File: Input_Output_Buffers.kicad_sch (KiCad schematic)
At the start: 35 parts, among them J1 Conn_02x07_Odd_Even, J4 Conn_02x07_Odd_Even, U1 74HC245, U2 74HC245, U26 74HC245, U27 74HC245

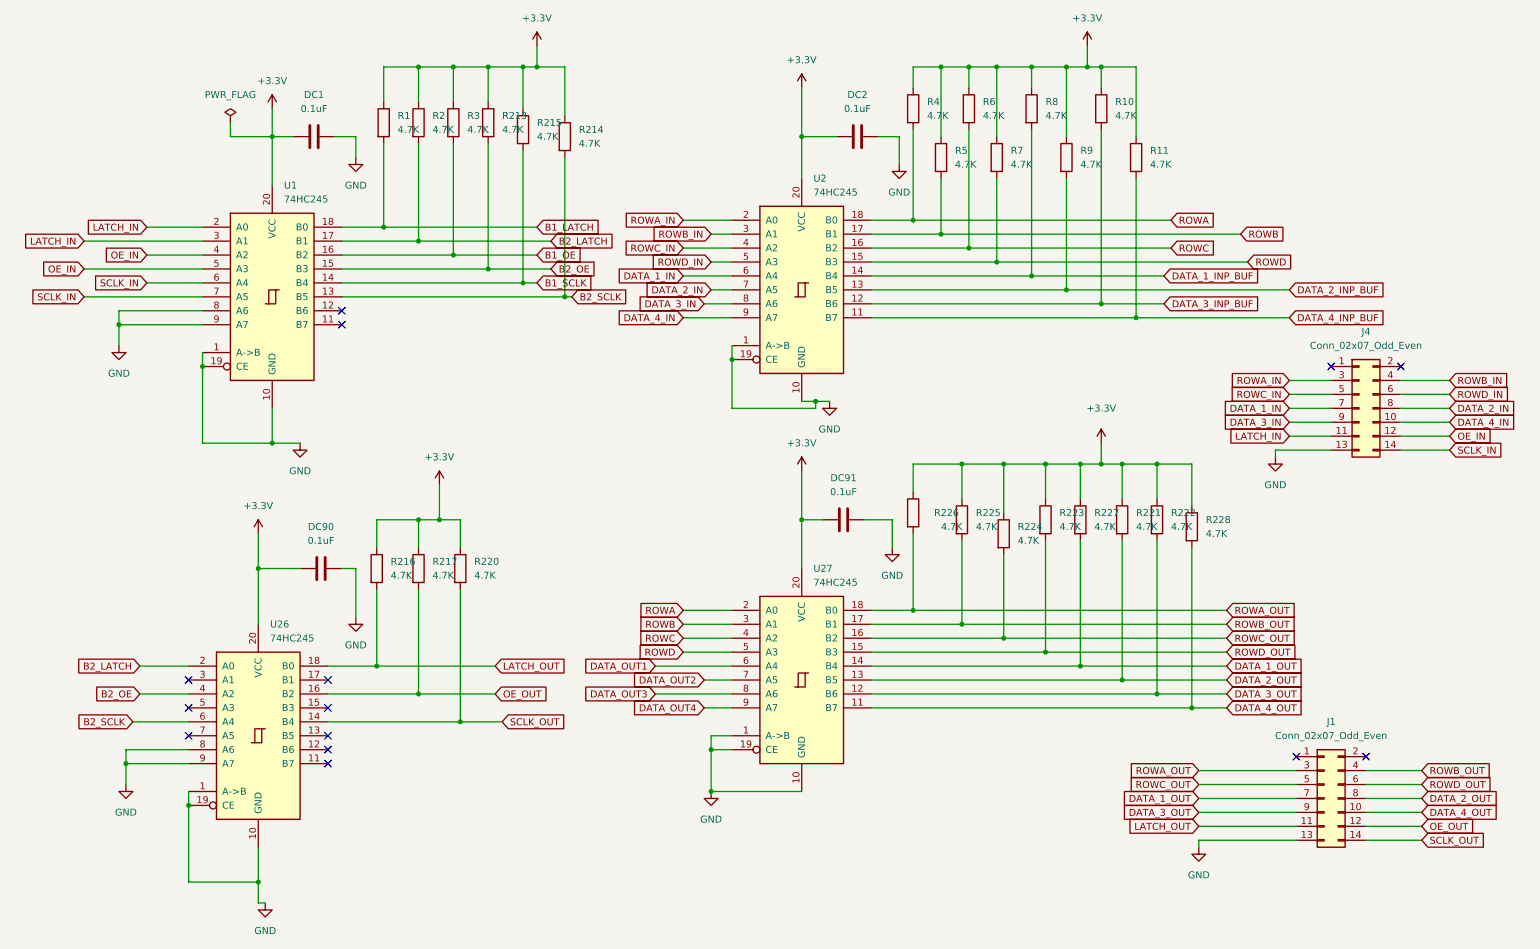
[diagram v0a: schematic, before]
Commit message: Updated PCB
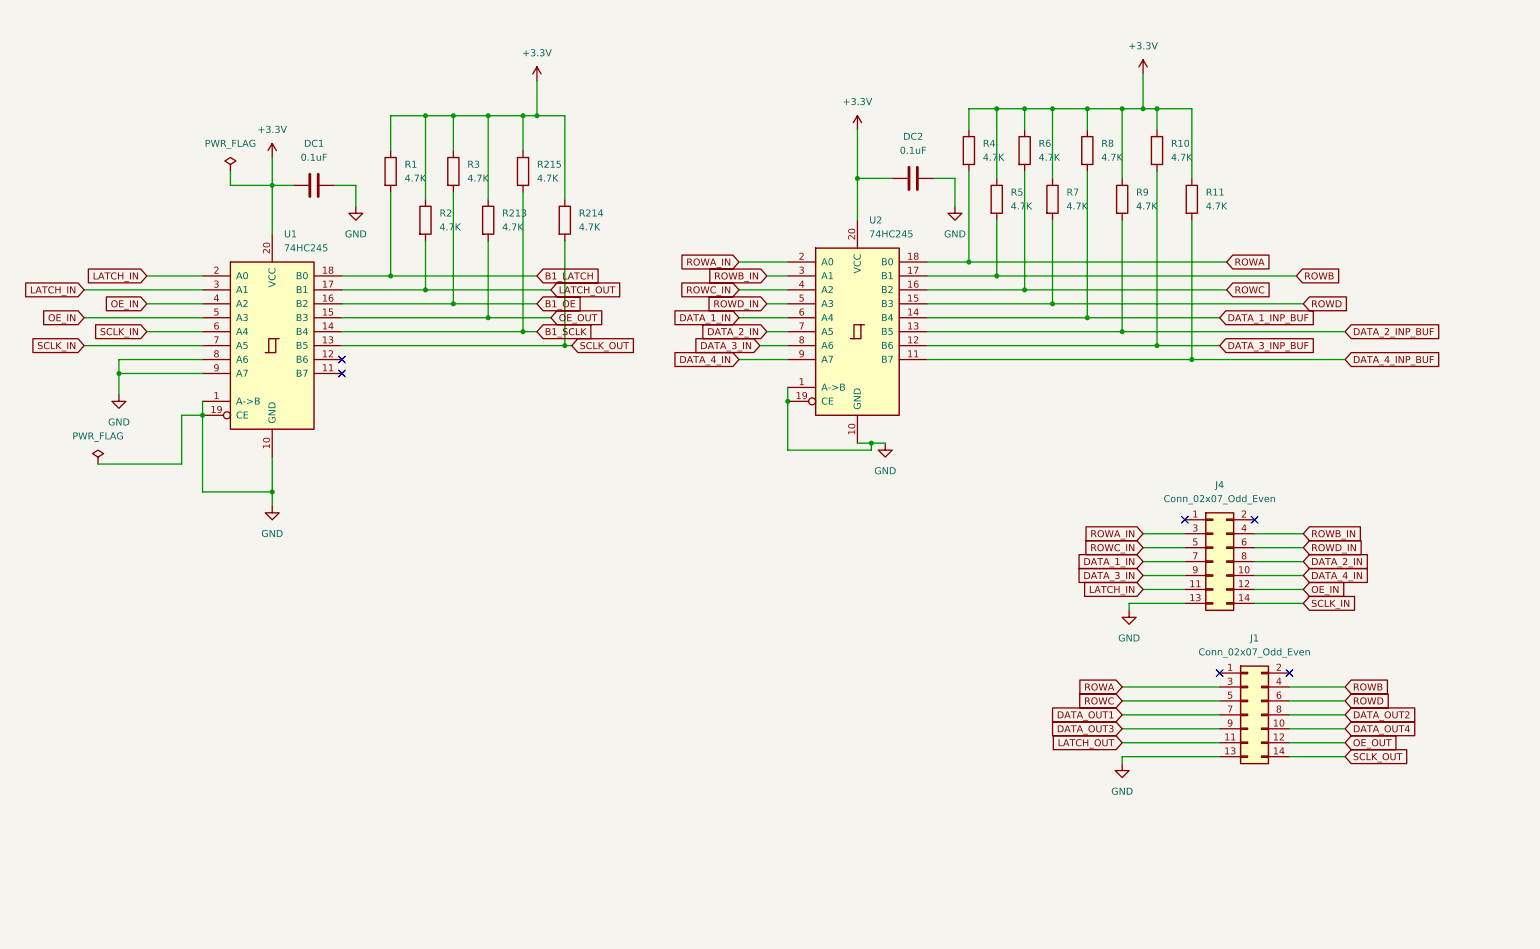
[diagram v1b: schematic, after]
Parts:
- removed DC90, DC91: 0.1uF, Capacitor_SMD:C_0805_2012Metric, symbol Device:C
- removed R216, R217, R220, R221, R222, R223, R224, R225, R226, R227, R228: 4.7K, Resistor_SMD:R_0805_2012Metric, symbol Device:R
- removed U26, U27: 74HC245, Package_SO:TSSOP-20_4.4x6.5mm_P0.65mm, symbol 74xx:74HC245
- U1, U2: footprint Package_SO:TSSOP-20_4.4x6.5mm_P0.65mm -> (none)
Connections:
- net B2_LATCH is gone; now on net LATCH_OUT: R2.2, U1.17 (B1)
- net B2_OE is gone; now on net OE_OUT: R213.2, U1.15 (B3)
- net B2_SCLK is gone; now on net SCLK_OUT: R214.2, U1.13 (B5)
- net DATA_1_OUT is gone; now on net DATA_OUT1: J1.7 (Pin_7)
- net DATA_2_OUT is gone; now on net DATA_OUT2: J1.8 (Pin_8)
- net DATA_3_OUT is gone; now on net DATA_OUT3: J1.9 (Pin_9)
- net DATA_4_OUT is gone; now on net DATA_OUT4: J1.10 (Pin_10)
- net ROWA_OUT is gone; now on net ROWA: J1.3 (Pin_3)
- net ROWB_OUT is gone; now on net ROWB: J1.4 (Pin_4)
- net ROWC_OUT is gone; now on net ROWC: J1.5 (Pin_5)
- net ROWD_OUT is gone; now on net ROWD: J1.6 (Pin_6)
- no-connect marks 14 -> 6
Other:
- moved on the sheet: DC1, DC2, J1, J4, R1, R10, R11, R2, R213, R214, R215, R3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
